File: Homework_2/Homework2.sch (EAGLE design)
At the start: 22 parts

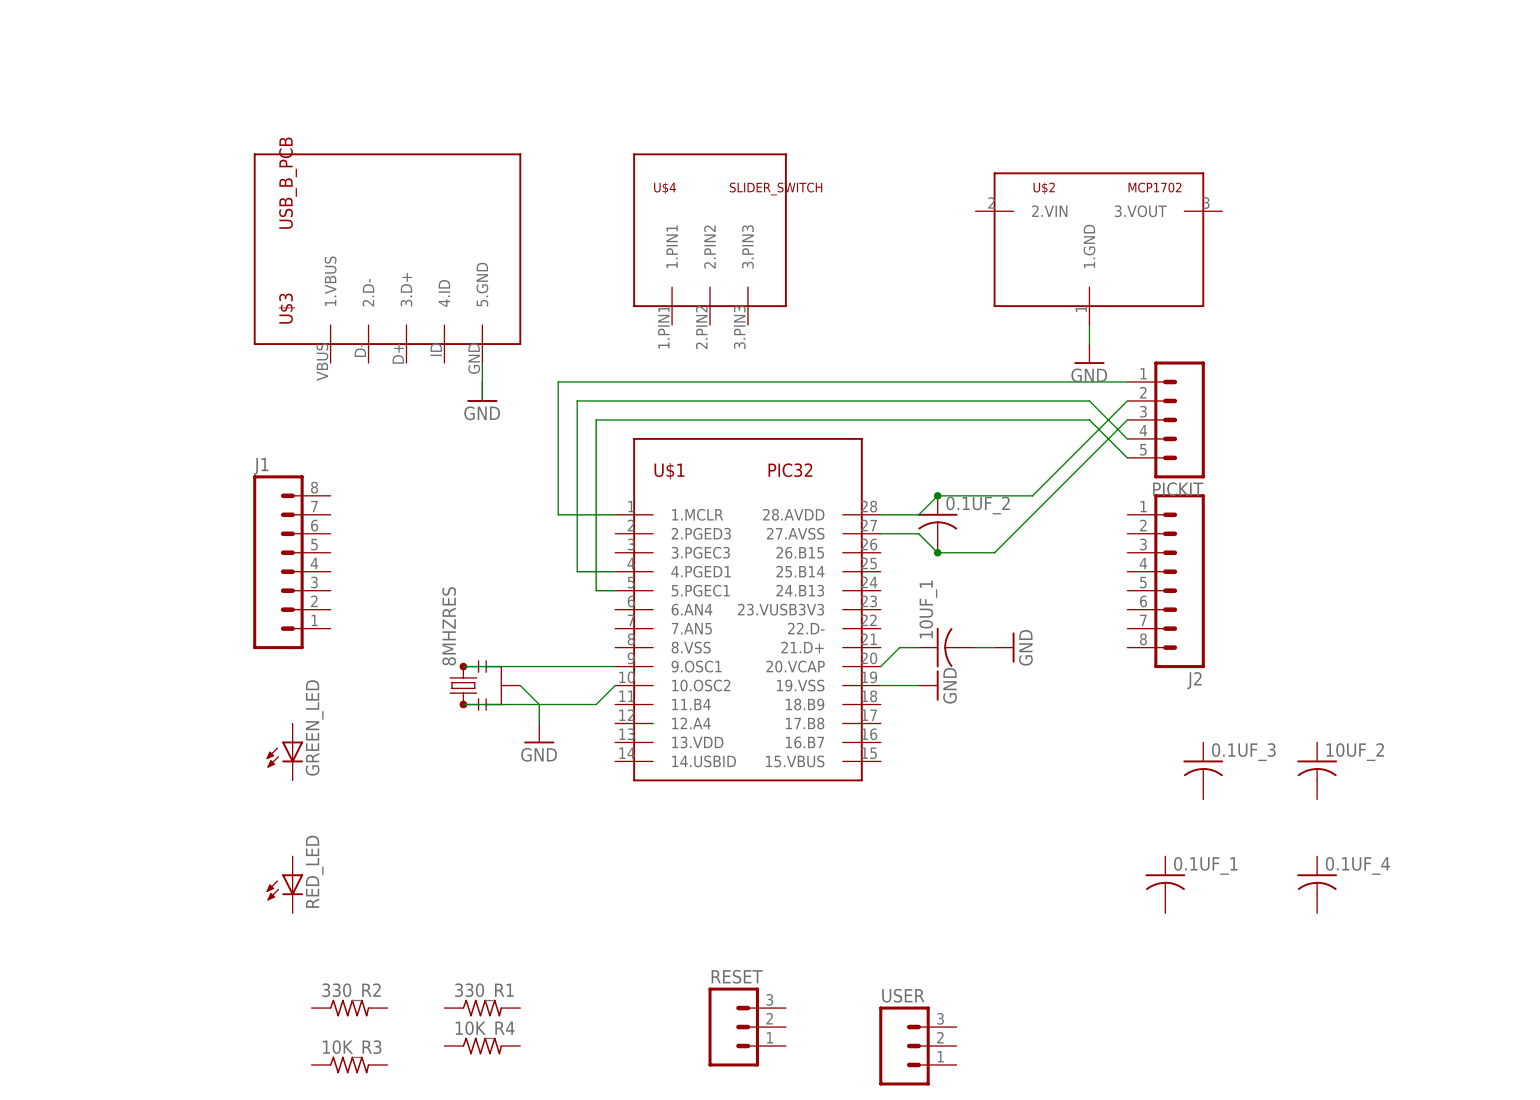
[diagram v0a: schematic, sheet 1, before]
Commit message: Homework_2/3_commit#5
finished schematic
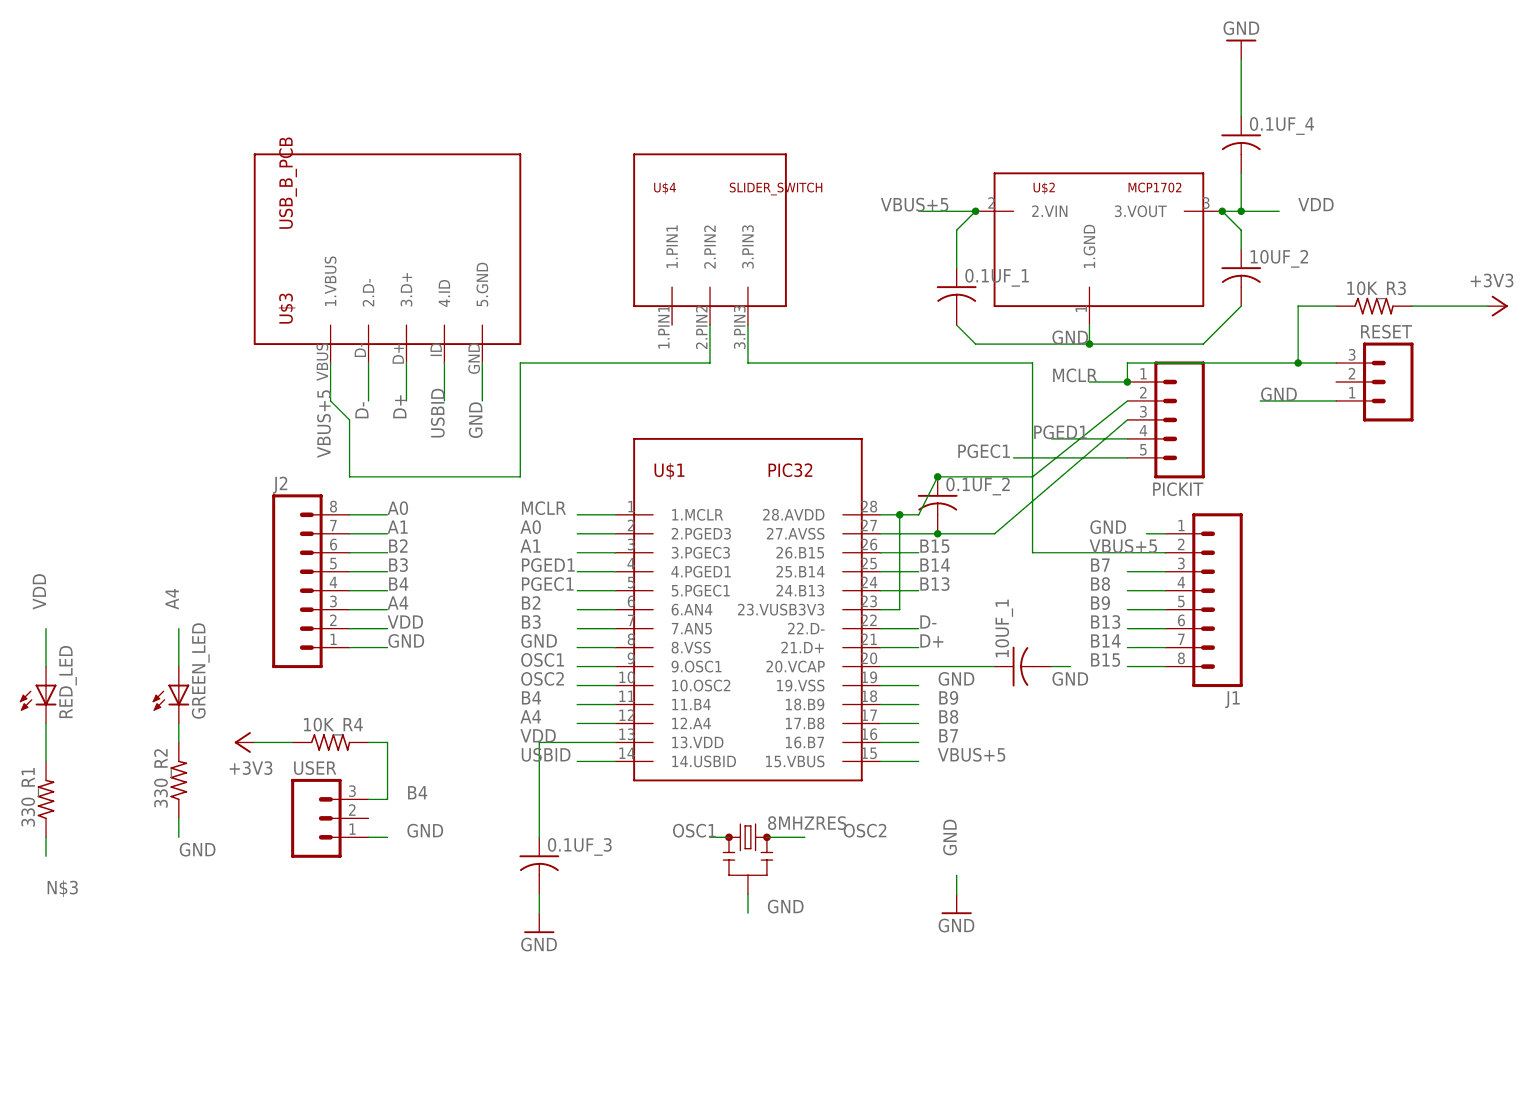
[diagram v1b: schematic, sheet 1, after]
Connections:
- net N$6 renamed PGED1
- net N$7 renamed PGEC1
- removed net N$4: U$3.5.GND
- removed net N$5: PICKIT.1, U$1.1.MCLR
- new net +3V3: 10K_R3.2, 10K_R4.1
- new net A0: J2.8, U$1.2.PGED3
- new net A1: J2.7, U$1.3.PGEC3
- new net A4: GREEN_LED.A, J2.3, U$1.12.A4
- new net B13: J1.6, U$1.24.B13
- new net B14: J1.7, U$1.25.B14
- new net B15: J1.8, U$1.26.B15
- new net B2: J2.6, U$1.6.AN4
- new net B3: J2.5, U$1.7.AN5
- new net B4: 10K_R4.2, J2.4, U$1.11.B4, USER.3
- new net B7: J1.3, U$1.16.B7
- new net B8: J1.4, U$1.17.B8
- new net B9: J1.5, U$1.18.B9
- new net D+: U$1.21.D+, U$3.3.D+
- new net D-: U$1.22.D-, U$3.2.D-
- new net MCLR: 10K_R3.1, PICKIT.1, RESET.3, U$1.1.MCLR
- new net N$3: 330_R1.1
- new net OSC1: 8MHZRES.1, U$1.9.OSC1
- new net OSC2: 8MHZRES.3, U$1.10.OSC2
- new net USBID: U$1.14.USBID, U$3.4.ID
- new net VBUS+5: 0.1UF_1.1, J1.2, U$1.15.VBUS, U$2.2.VIN, U$3.1.VBUS, U$4.2.PIN2, U$4.3.PIN3
- new net VDD: 0.1UF_3.1, 0.1UF_4.2, 10UF_2.1, J2.2, RED_LED.A, U$1.13.VDD, U$2.3.VOUT
- net GND: now also 0.1UF_1.2, 0.1UF_3.2, 0.1UF_4.1, 10UF_2.2, 330_R2.1, J1.1, J2.1, RESET.1, U$1.8.VSS, U$3.5.GND, USER.1
- net N$1: now also 330_R2.2, GREEN_LED.C; no longer 8MHZRES.3, U$1.9.OSC1
- net N$2: now also 330_R1.2, RED_LED.C; no longer 8MHZRES.1, U$1.10.OSC2
- net N$9: now also U$1.23.VUSB3V3
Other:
- moved on the sheet: 0.1UF_1, 0.1UF_2, 0.1UF_3, 0.1UF_4, 10K_R3, 10K_R4, 10UF_1, 10UF_2, 330_R1, 330_R2, 8MHZRES, GREEN_LED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
